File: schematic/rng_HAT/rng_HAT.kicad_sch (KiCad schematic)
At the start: 32 parts, among them J1 RPi_GPIO, Q1 2N3904, Q2 2N3904, Q3 2N3904, Q4 BC107, Q5 2N3904, U3 STM32F103C8Tx

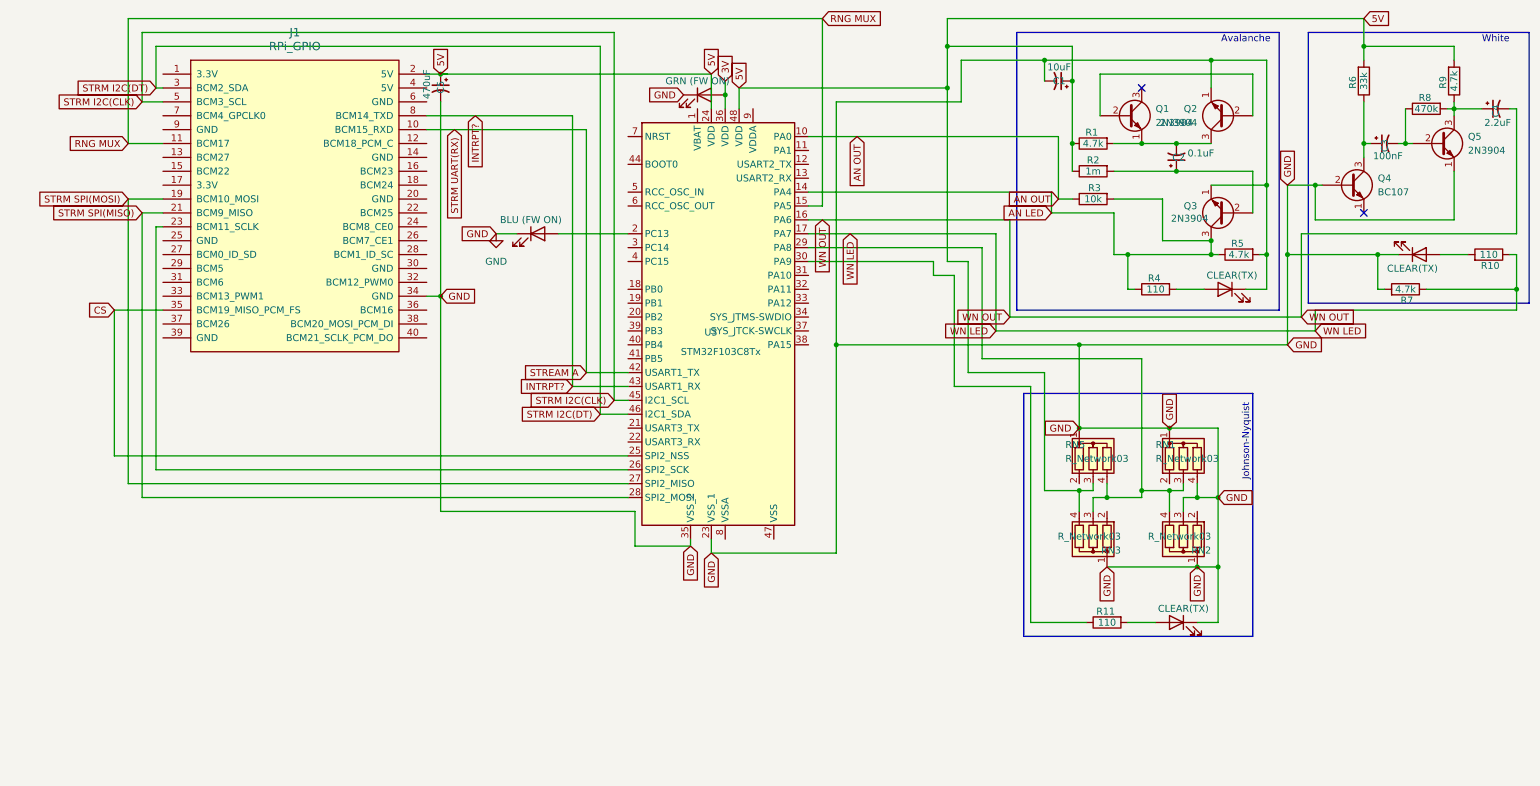
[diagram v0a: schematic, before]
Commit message: some more PCB updates
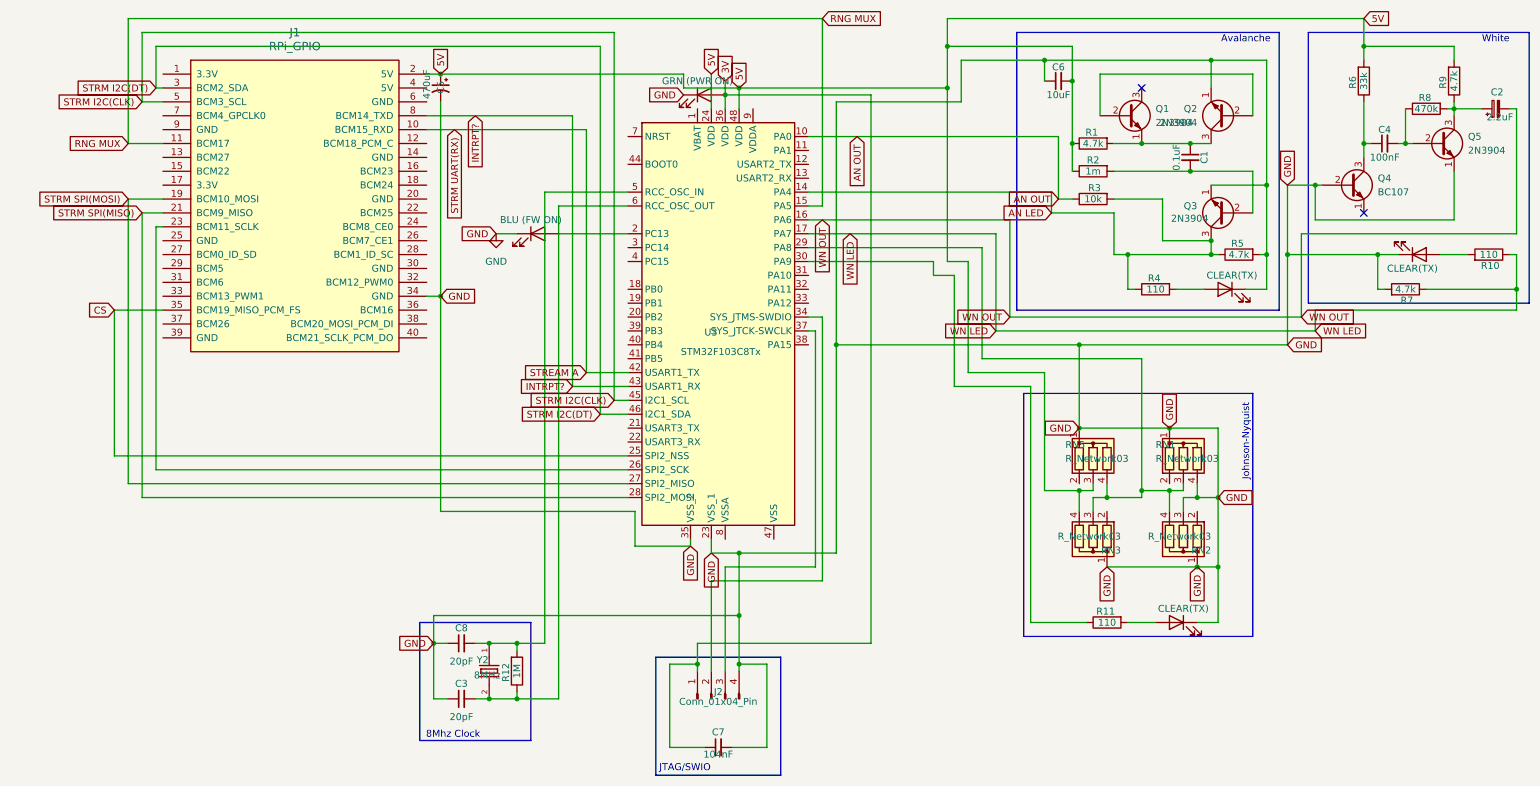
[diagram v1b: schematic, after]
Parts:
- removed C1: 10uF, Capacitor_SMD:CP_Elec_3x5.3, symbol Device:C_Polarized_Small_US
- removed C2: 0.1uF, Capacitor_SMD:CP_Elec_3x5.3, symbol Device:C_Polarized_Small_US
- removed C3: 100nF, Capacitor_SMD:CP_Elec_3x5.3, symbol Device:C_Polarized_Small_US
- removed C4: 2.2uF, Capacitor_SMD:CP_Elec_3x5.3, symbol Device:C_Polarized_Small_US
- added C1: 0.1uF, Capacitor_SMD:C_0603_1608Metric_Pad1.08x0.95mm_HandSolder, symbol Device:C_Small
- added C2: 2.2uF, Capacitor_SMD:C_0603_1608Metric_Pad1.08x0.95mm_HandSolder, symbol Device:C_Polarized_Small
- added C3, C8: 20pF, Capacitor_SMD:C_0603_1608Metric_Pad1.08x0.95mm_HandSolder, symbol Device:C_Small
- added C4: 100nF, Capacitor_SMD:C_0603_1608Metric_Pad1.08x0.95mm_HandSolder, symbol Device:C_Small
- added C6: 10uF, Capacitor_SMD:C_0603_1608Metric_Pad1.08x0.95mm_HandSolder, symbol Device:C_Small
- added C7: 104nF, Capacitor_SMD:C_0603_1608Metric_Pad1.08x0.95mm_HandSolder, symbol Device:C_Small
- added J2: Conn_01x04_Pin, Connector_PinHeader_1.00mm:PinHeader_1x04_P1.00mm_Horizontal, symbol Connector:Conn_01x04_Pin
- added R12: 1M, Resistor_SMD:R_0201_0603Metric, symbol Device:R
- added Y2: 8MHz, Crystal:Crystal_SMD_3215-2Pin_3.2x1.5mm, symbol ECS-80-S-4X:ECS-80-S-4X
- D4: value GRN (FW ON) -> GRN (PWR ON)
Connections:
- net 3V: now also C7.1, J2.1 (Pin_1)
- net 5V: now also C6.2
- net GND: now also C3.1, C6.1, C7.2, C8.1, J2.4 (Pin_4)
- net WN OUT: now also C2.2
- net at Q5.2 (B), R8.1: now also C4.2
- net at Q5.3 (C), R8.2, R9.1: now also C2.1
- net at Q3.2 (B), R2.2: now also C1.2
- net at Q1.1 (E), Q2.3 (C), R1.2: now also C1.1
- net at Q4.3 (C), R6.1: now also C4.1
- net at U3.34 (PA13): now also J2.2 (Pin_2)
- net at U3.37 (PA14): now also J2.3 (Pin_3)
- net at U3.5 (PD0): now also C8.2, R12.2, Y2.1
- net at U3.6 (PD1): now also C3.2, R12.1, Y2.2
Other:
- note added: "8Mhz Clock"
- note added: "JTAG/SWIO"
